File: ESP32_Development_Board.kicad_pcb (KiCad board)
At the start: 4 copper layers, 70 x 20.3 mm, 47 parts, among them J1 Conn_01x17_Pin, J2 Conn_01x17_Pin, J3 Conn_01x03_Pin, J4 USB_B_Micro, J5 Conn_01x02_Pin, Q1 NPN, Q2 NPN, Q3 Q_NMOS_GDS, Q4 Q_NMOS_GDS, SW1 SW_Push, SW2 SW_Push, U1 ESP32-WROOM-32E, U2 CP2102N-Axx-xQFN28, U3 AMS1117-3.3

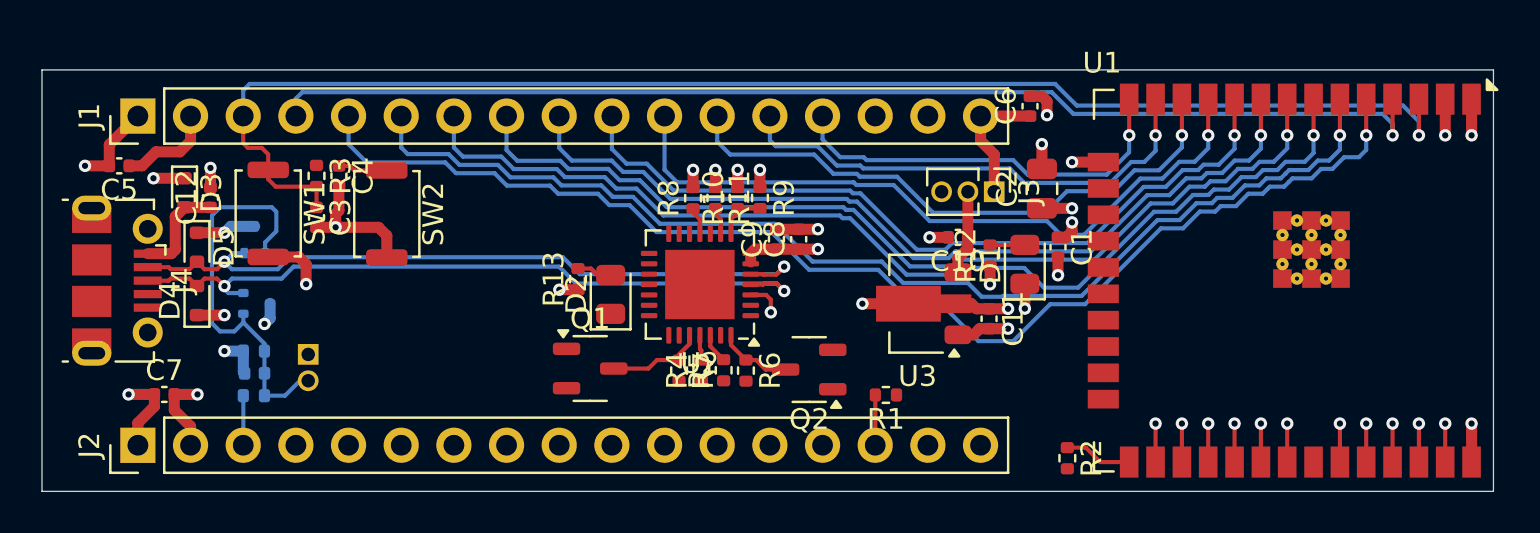
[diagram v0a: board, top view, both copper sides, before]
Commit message: Commit at 2025-08-20 20:00:00
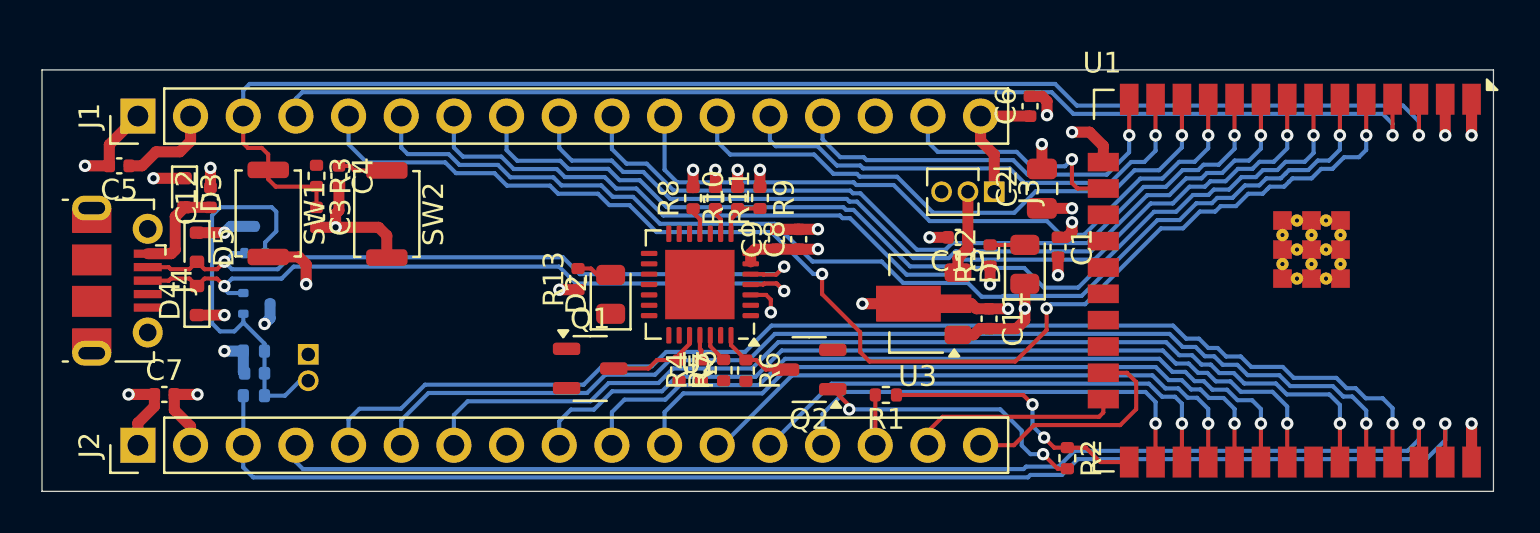
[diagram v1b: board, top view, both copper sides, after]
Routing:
- net /IO23: track 4.25 -> 65.0 mm
- net /IO22: track 1.86 -> 58.3 mm
- net /TXD0: track 1.86 -> 57.7 mm
- net /RXD0: track 1.86 -> 53.5 mm
- net /IO21: track 1.86 -> 49.7 mm
- net /IO19: track 1.86 -> 41.5 mm
- net /IO18: track 1.86 -> 37.5 mm
- net /IO5: track 1.86 -> 33.4 mm
- net /IO17: track 1.86 -> 28.3 mm
- net /IO16: track 1.86 -> 24.3 mm
- net /IO4: track 1.86 -> 21.1 mm
- net /IO0_BTN: track 2.40 -> 15.8 mm, vias 0 -> 2
- net /IO13: track 0.00 -> 11.6 mm, vias 0 -> 1
- net /IO15: track 0.00 -> 11.3 mm
- net /IO2: track 0.00 -> 10.1 mm
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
